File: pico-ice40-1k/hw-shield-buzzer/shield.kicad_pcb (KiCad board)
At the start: 2 copper layers, 53.3 x 53.8 mm, 30 parts, among them J1 JACK_TRS_6PINS, P1 CONN_12, P2 CONN_12, P3 CONN_01X02, SW2 SW_PUSH, U1 TLV320DAC3203, U2 LD39015M18R, U3 TPA2005D1

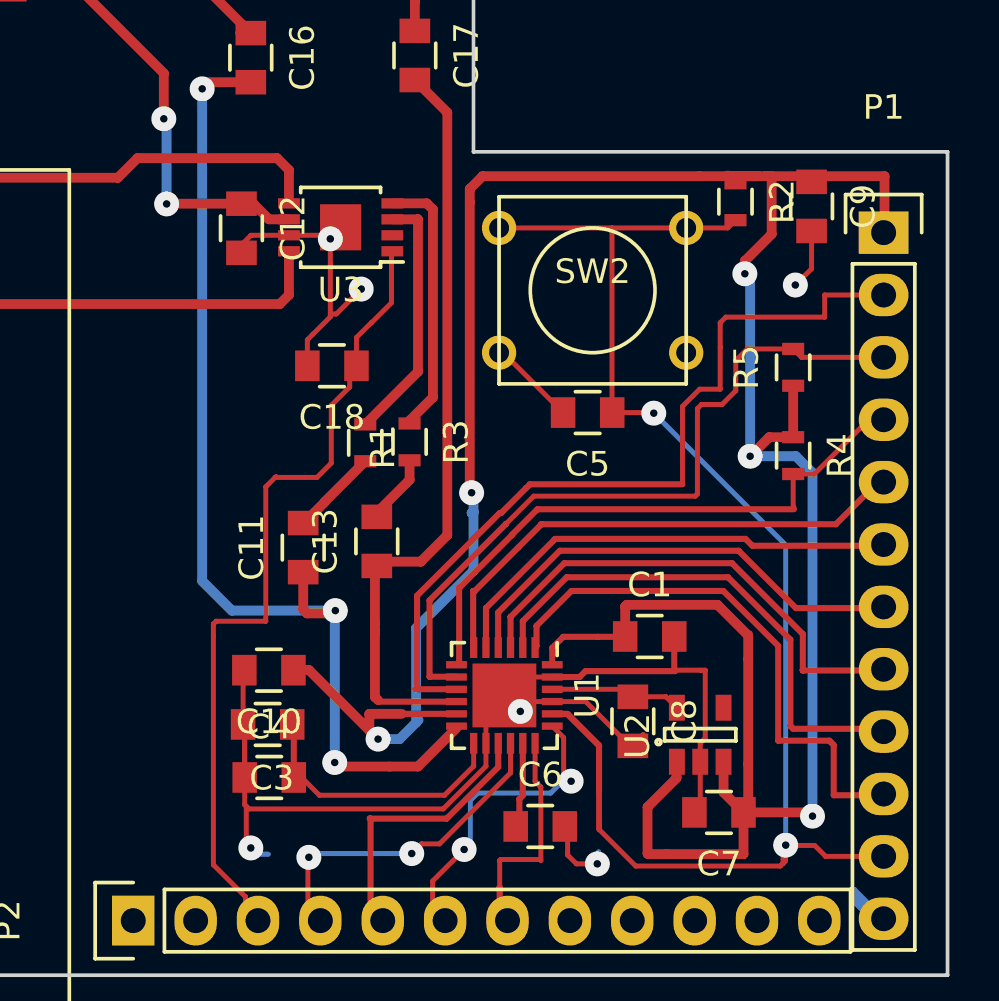
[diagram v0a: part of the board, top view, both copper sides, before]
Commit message: Small changes on the pcb
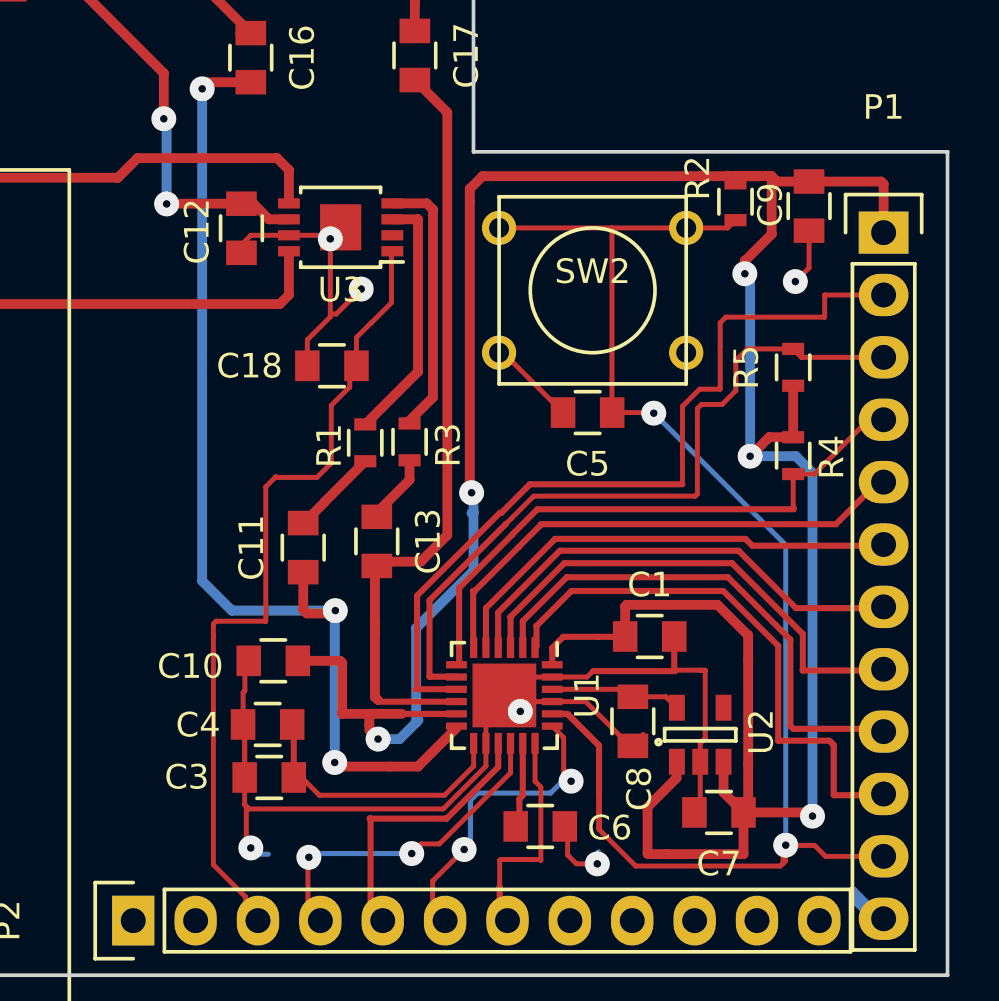
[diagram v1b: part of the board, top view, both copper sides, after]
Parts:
- moved C10 0.42 mm to (171.7, 91.3)
- moved C9 0.10 mm to (193.5, 72.8)
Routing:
- net GND: track 78.0 -> 83.5 mm
